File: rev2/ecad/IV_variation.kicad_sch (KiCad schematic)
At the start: 35 parts, among them Q1 IRF3205, Q2 IRF4905, Q5 IRF3205, Q6 IRF4905, U2 LM6144xIx

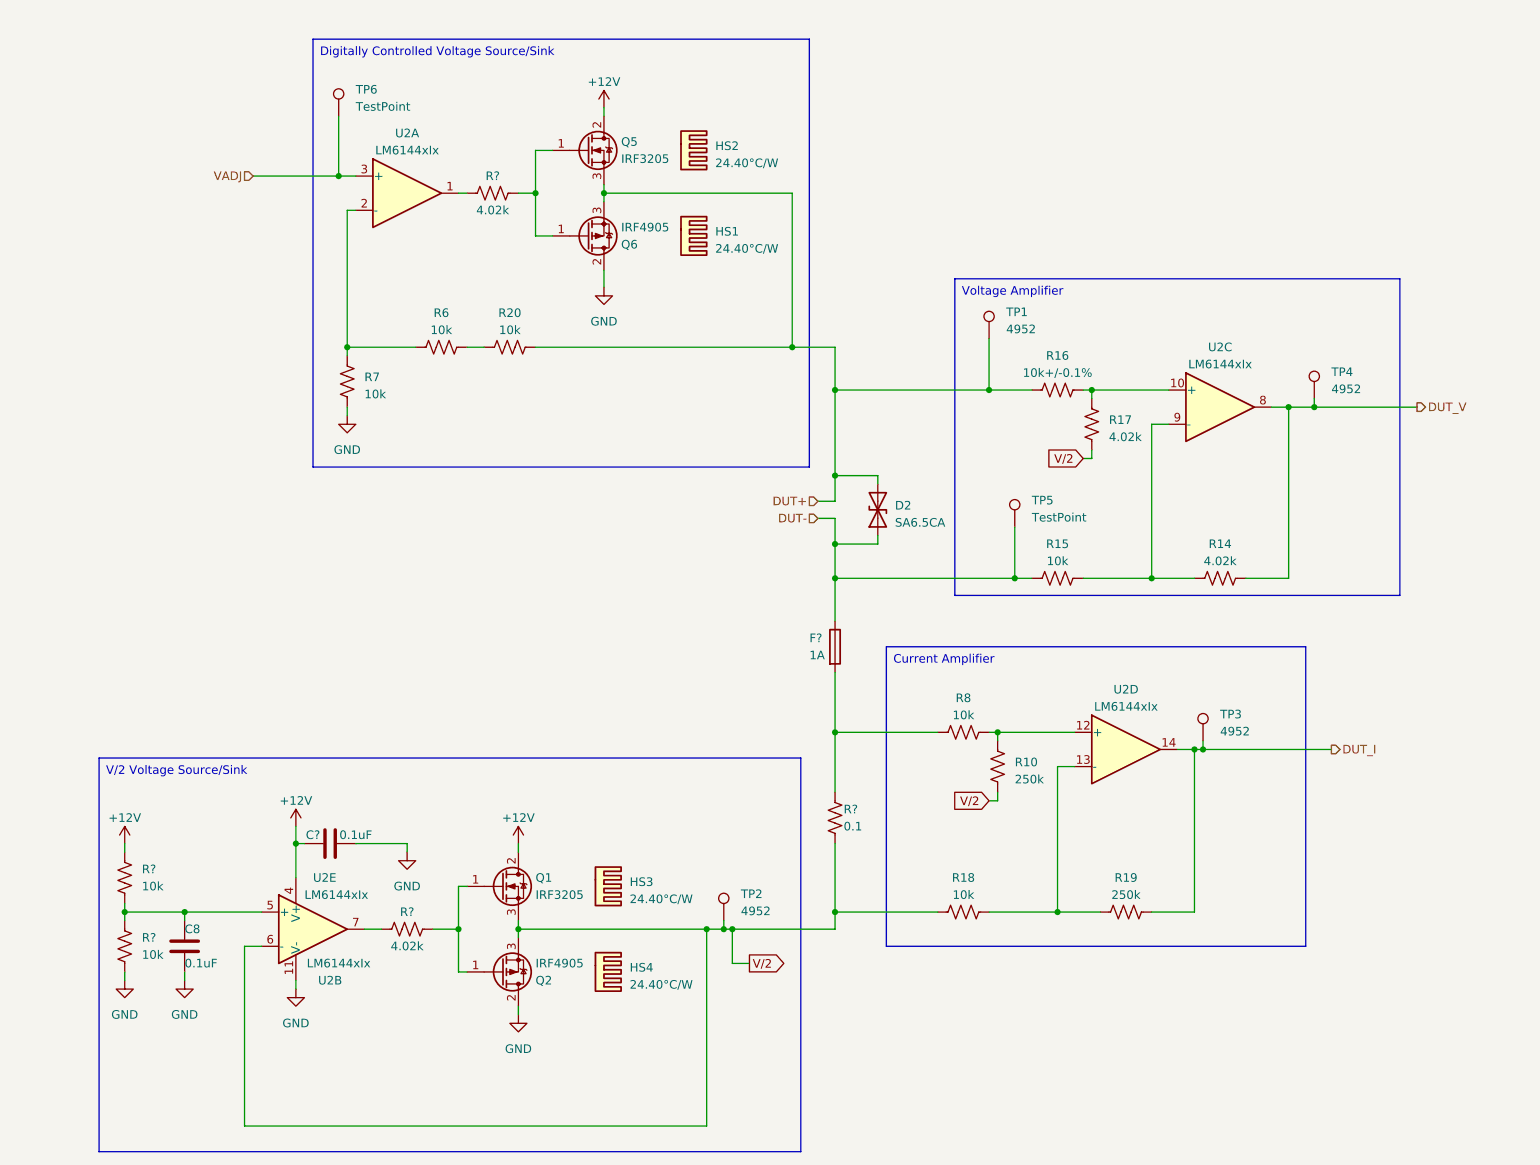
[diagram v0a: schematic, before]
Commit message: layout
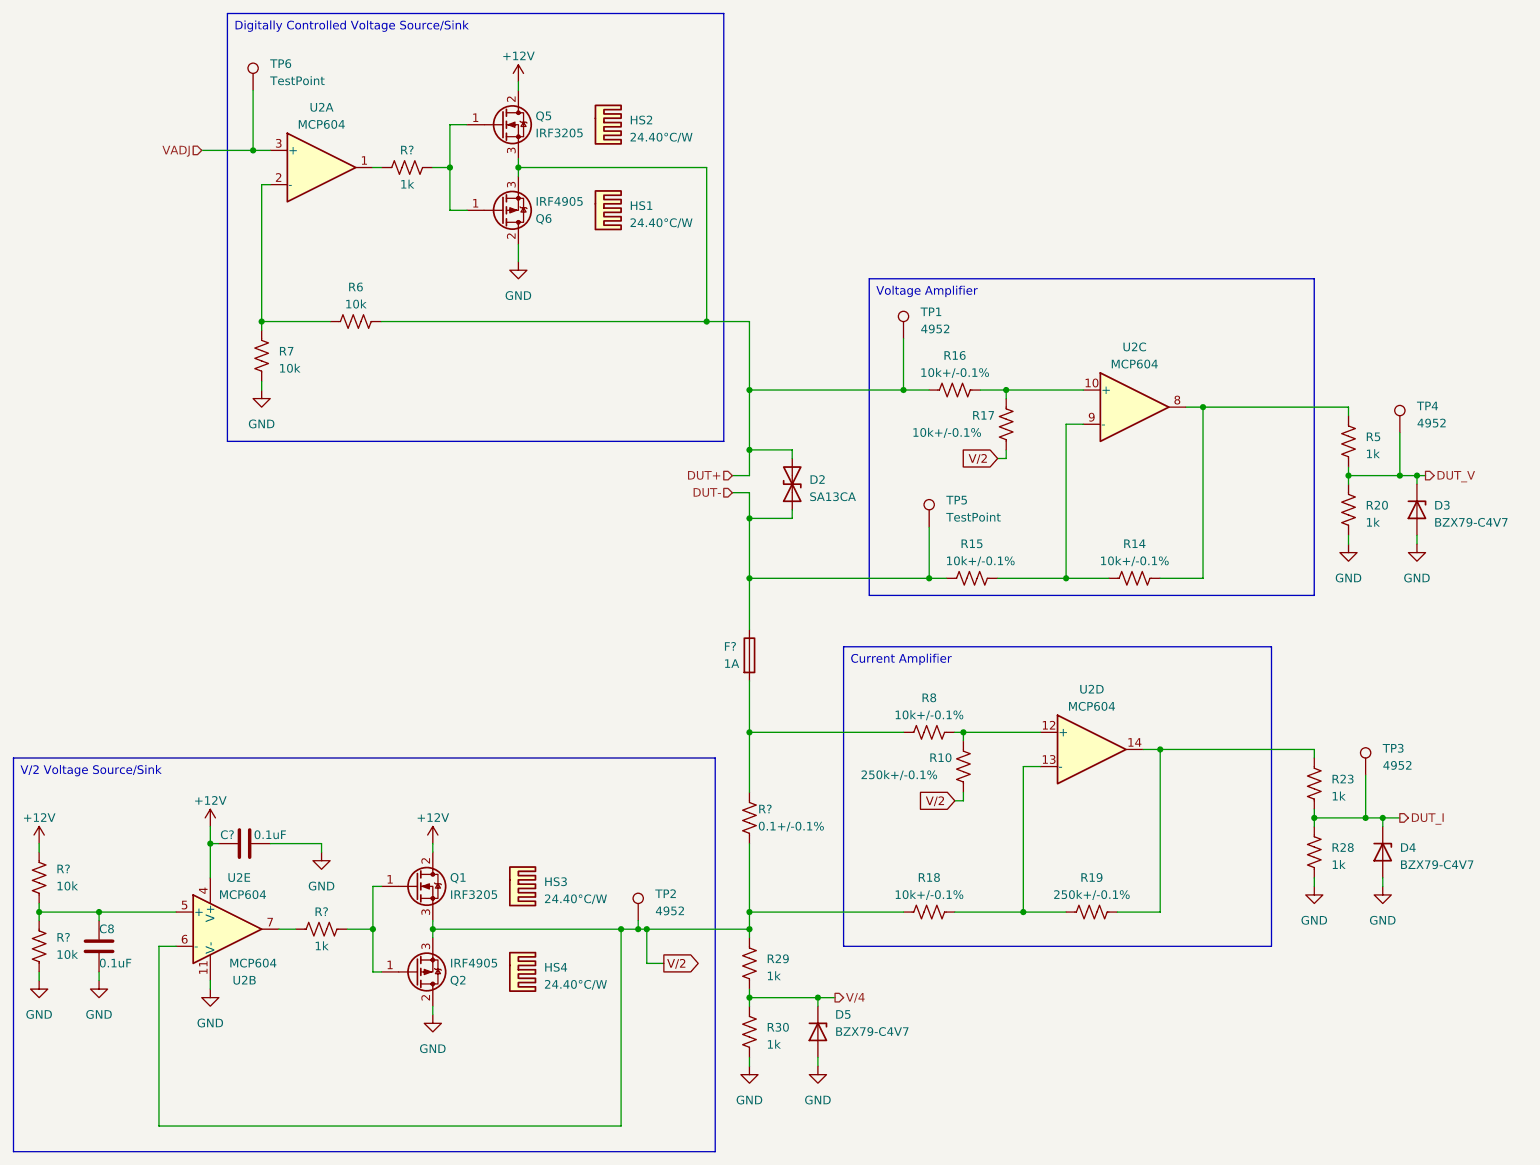
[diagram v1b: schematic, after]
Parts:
- added D3, D4, D5: BZX79-C4V7, Diode_THT:D_DO-35_SOD27_P7.62mm_Horizontal, symbol Device:D_Zener
- added R23, R28, R29, R30, R5: 1k, Resistor_THT:R_Axial_DIN0207_L6.3mm_D2.5mm_P7.62mm_Horizontal, symbol Device:R_US
- D2: value SA6.5CA -> SA13CA
- R10, R19: value 250k -> 250k+/-0.1%
- R14, R17: value 4.02k -> 10k+/-0.1%
- R15, R18, R8: value 10k -> 10k+/-0.1%
- R20: value 10k -> 1k
- R? (x2): value 4.02k -> 1k
- R?: value 0.1 -> 0.1+/-0.1%
- U2: value LM6144xIx -> MCP604
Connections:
- net DUT+: now also R6.2; no longer R20.2
- net DUT_I: now also D4.1 (K), R23.2, R28.1; no longer R19.2, U2.14
- net DUT_V: now also R20.1, D3.1 (K), R5.2; no longer R14.2, U2.8
- net GND: now also R20.2, D3.2 (A), D4.2 (A), D5.2 (A), R28.2, R30.2
- net V/2: now also R29.1
- new net: R19.2, R23.1, U2.14
- new net: R14.2, R5.1, U2.8
- new net V/4: D5.1 (K), R29.2, R30.1
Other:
- title: Analog IV Variation -> Analog Front End
- moved on the sheet: C8, C?, D2, F?, HS1, HS2, HS3, HS4, Q1, Q2, Q5, Q6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
